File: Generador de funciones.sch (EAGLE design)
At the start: 41 parts, among them IC1 ICL8038, IC2 TL084P, IC3 LF353N

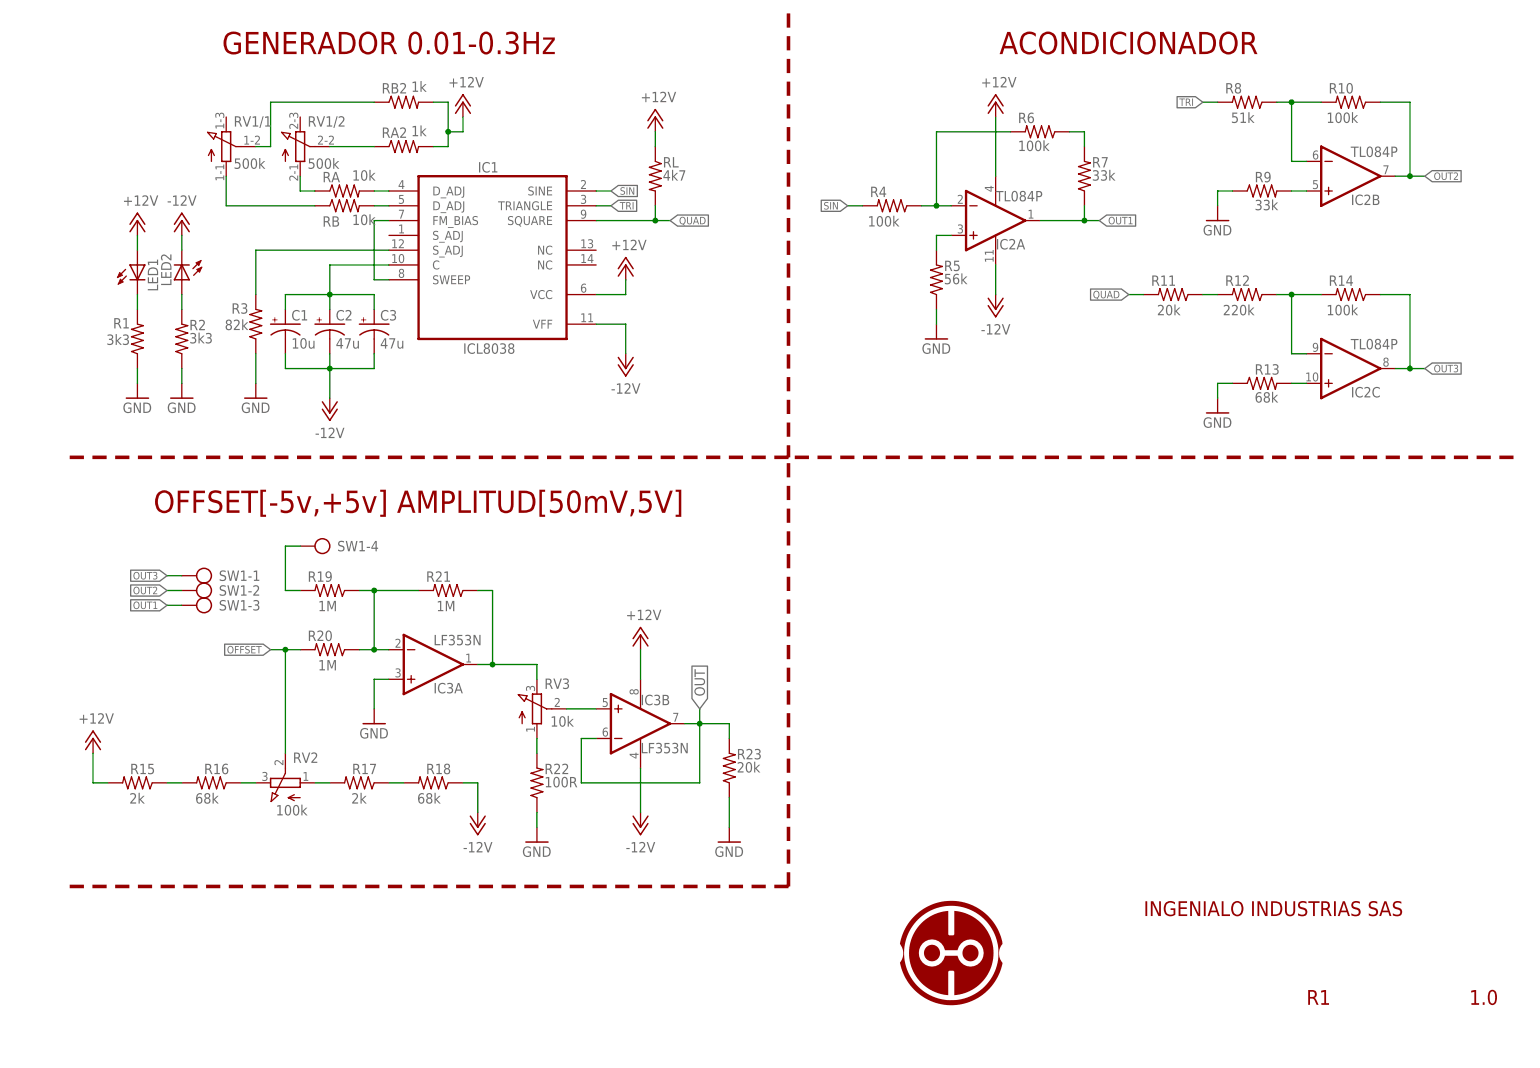
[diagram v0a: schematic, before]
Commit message: Generado imagenes SCH y BRD
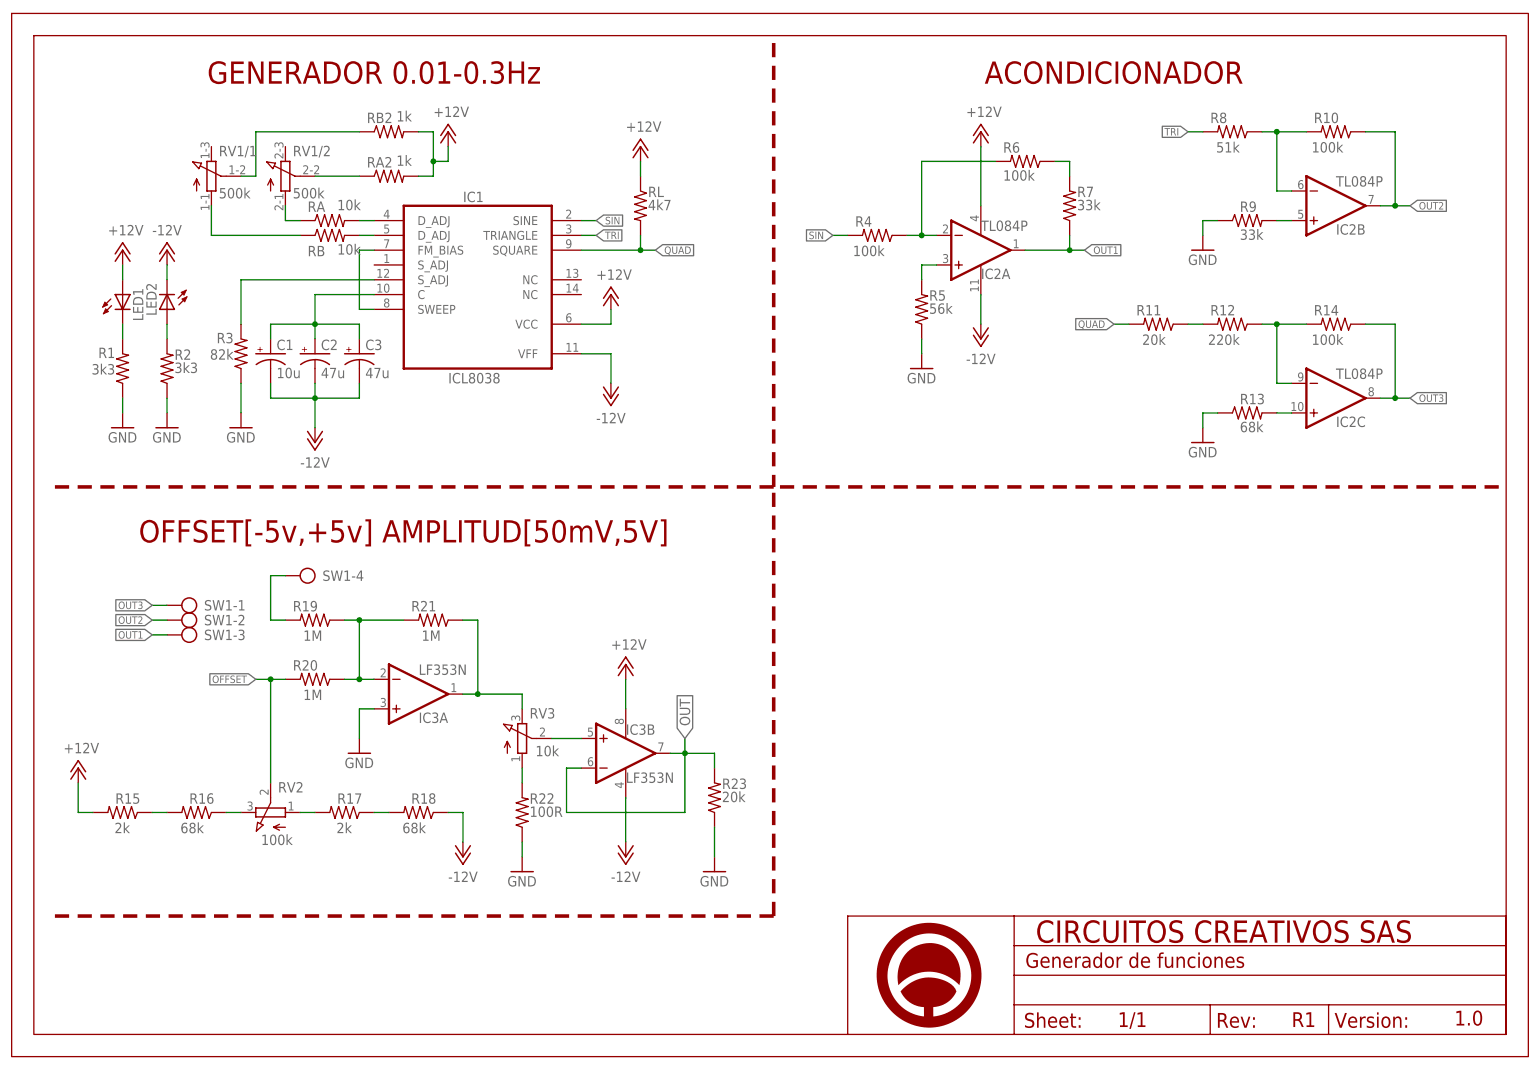
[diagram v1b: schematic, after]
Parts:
- removed U$1: LOGO_REDUCIDO, Ingenialo_logos:LOGO_REDUCIDO
- added FRAME1: A4_HORIZONTAL, Circuitos-Creativos-Estilos:A4_HORIZONTAL
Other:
- note removed: "INGENIALO INDUSTRIAS SAS"
- moved on the sheet: C1, C2, C3, IC1, IC2A, IC2B, IC2C, IC3A, IC3B, LED1, LED2, R1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
